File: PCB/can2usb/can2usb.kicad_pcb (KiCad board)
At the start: 2 copper layers, 39 parts, among them J1 STLINK, J2 Conn_01x03_Male, P1 USB_C_Plug_USB2.0, U1 STM32F103C6Tx, U2 TLP175A, U3 MCP2561-E-SN, U5 USBLC6-2SC6, U6 MIC5528-3.3YMT-TR, Y1 16MHz, Y2 32KHz

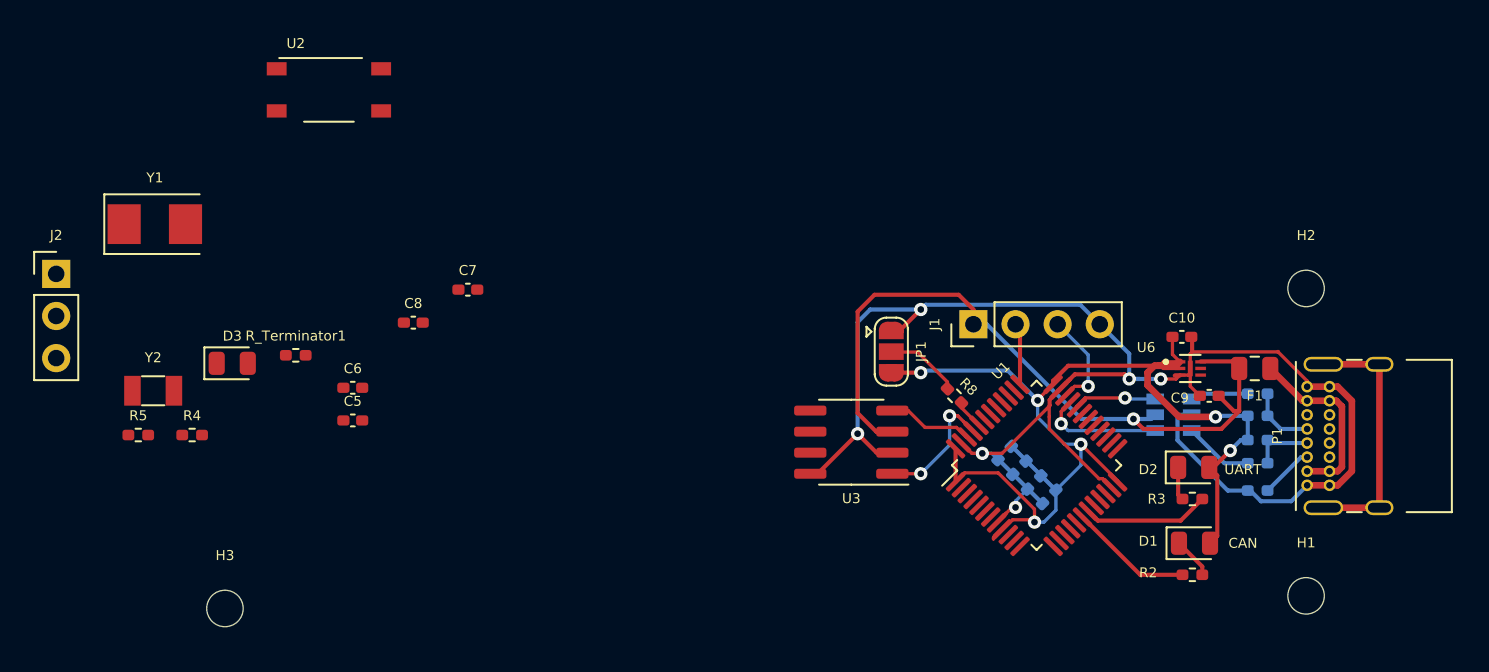
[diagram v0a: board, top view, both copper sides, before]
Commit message: New PCB design
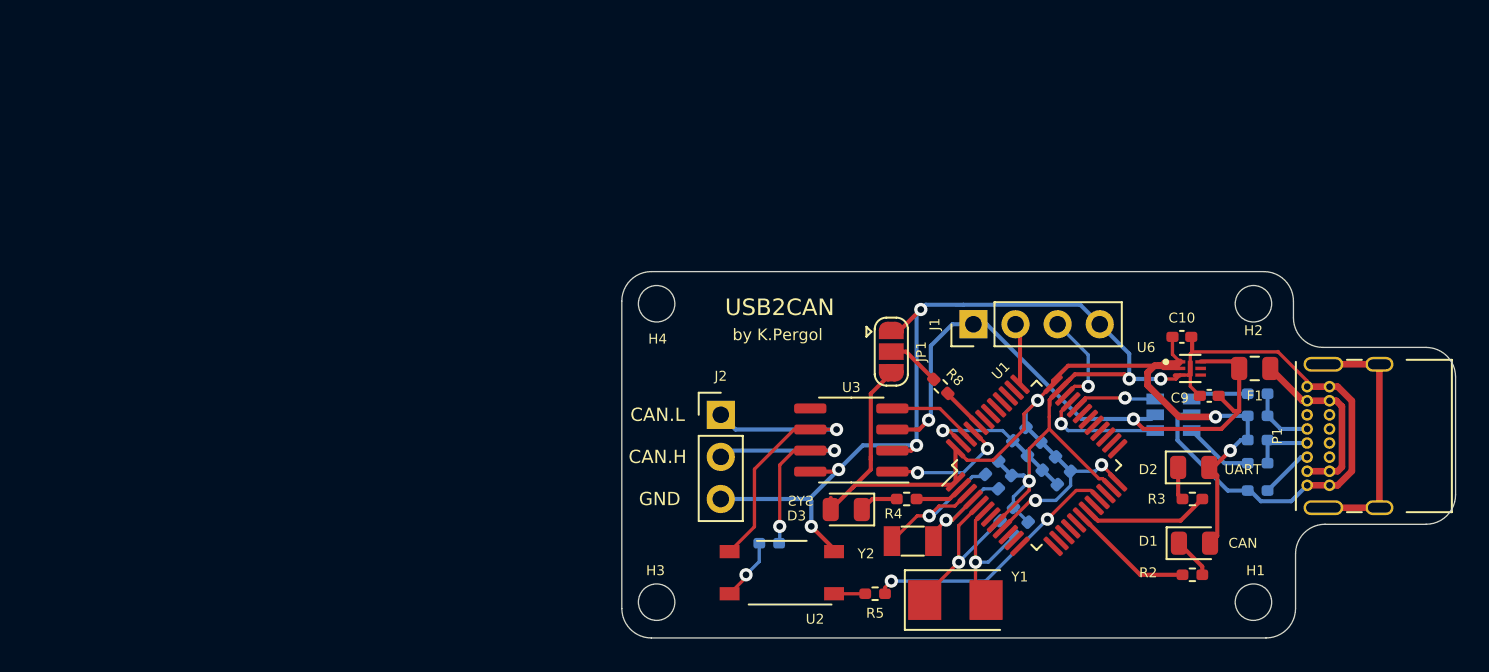
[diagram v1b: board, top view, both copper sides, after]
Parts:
- added H4: MountingHole, MountingHole:MountingHole_2.2mm_M2, F.Cu at (112.3, 73.1)
- C5, C6, C7, C8, R_Terminator1: moved to B.Cu
- moved Y1 53.3 mm to (130.4, 90.9)
- moved Y2 46.7 mm to (127.8, 87.4), turned to 180 degrees
- moved R5 45.5 mm to (125.5, 90.6), turned to 180 degrees
- moved R4 43.3 mm to (127.4, 84.8)
- moved C6 41.2 mm to (134.3, 86.6), turned to 45 degrees
- moved J2 41.0 mm to (116.2, 79.8)
- moved U2 39.9 mm to (119.9, 89.3), turned to 180 degrees
- moved C5 39.9 mm to (133.5, 85.7), turned to 45 degrees
- moved D3 38.1 mm to (123.8, 85.5), turned to 180 degrees
- moved C8 37.0 mm to (133.3, 83.8), turned to 45 degrees
- moved C7 33.4 mm to (132.6, 83.0), turned to 45 degrees
- moved R_Terminator1 30.7 mm to (119.1, 87.5), turned to 180 degrees
- moved H3 26.0 mm to (112.3, 91.1)
- moved H2 3.31 mm to (148.3, 73.1)
- moved H1 3.20 mm to (148.3, 91.1)
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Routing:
- net GND: track 103.6 -> 124.2 mm, vias 6 -> 8
- net CAN_L: track 0.00 -> 18.9 mm, vias 0 -> 1
- net TERMINATOR_SW: track 0.00 -> 16.2 mm, vias 0 -> 2
- net CAN_H: track 0.00 -> 15.4 mm, vias 0 -> 2
- net OSC_IN: track 0.00 -> 10.6 mm, vias 0 -> 1
- net L_OSC_IN: track 0.00 -> 10.2 mm, vias 0 -> 1
- net OSC_OUT: track 0.00 -> 8.90 mm, vias 0 -> 1
- net L_OSC_OUT: track 0.00 -> 7.67 mm, vias 0 -> 1
- net +5V: track 44.5 -> 37.3 mm, vias 1 -> 2
- net Net-(R_Terminator1-Pad2): track 0.00 -> 3.79 mm, vias 0 -> 1
- net B_LED: track 0.00 -> 2.99 mm
- net Net-(D3-Pad1): track 0.00 -> 2.37 mm
- net Net-(R5-Pad2): track 0.00 -> 1.88 mm
- net +3V3: track 72.1 -> 73.6 mm, vias 6 -> 5
- net Net-(JP1-Pad2): track 4.56 -> 3.29 mm
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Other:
- board outline added: 50.3 x 22.1 mm
- rule trace_min: 0.2 -> 0.1
- board text added: "CAN.H"
- board text added: "CAN.L"
- board text added: "GND"
- board text added: "SYS"
- board text added: "USB2CAN"
- board text added: "by K.Pergol"
